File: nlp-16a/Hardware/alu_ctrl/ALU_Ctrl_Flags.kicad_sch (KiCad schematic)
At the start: 18 parts, among them U1 CD74HC00, U10 CD74HC00, U11 CD74HC00, U12 CD74HC00, U13 CD74HC00, U14 CD74HC00, U15 CD74HC00, U16 CD74HC00, U17 CD74HC00, U18 CD74HC00, U2 CD74HC00, U3 CD74HC00, U4 CD74HC00, U5 CD74HC00, U6 CD74HC00, U7 CD74HC00, U8 CD74HC00, U9 CD74HC00

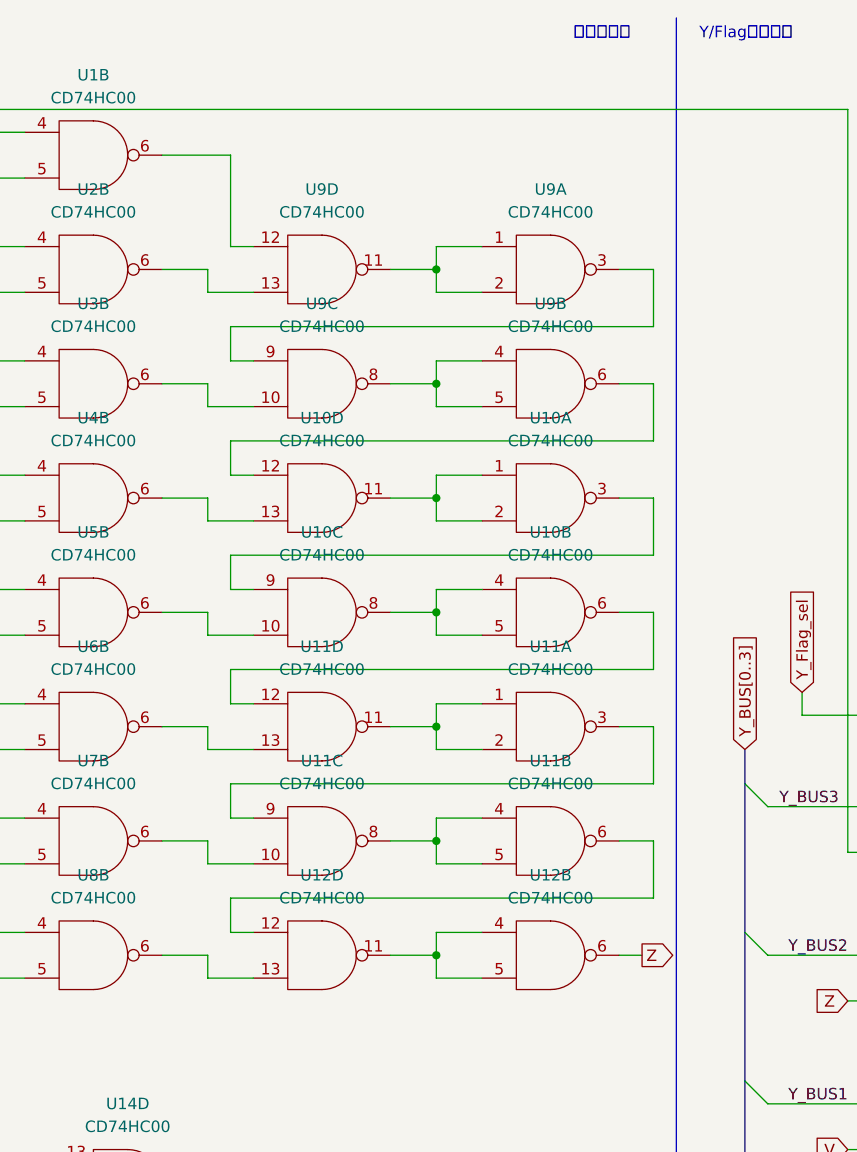
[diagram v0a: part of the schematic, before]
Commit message: ゼロフラグ高速化
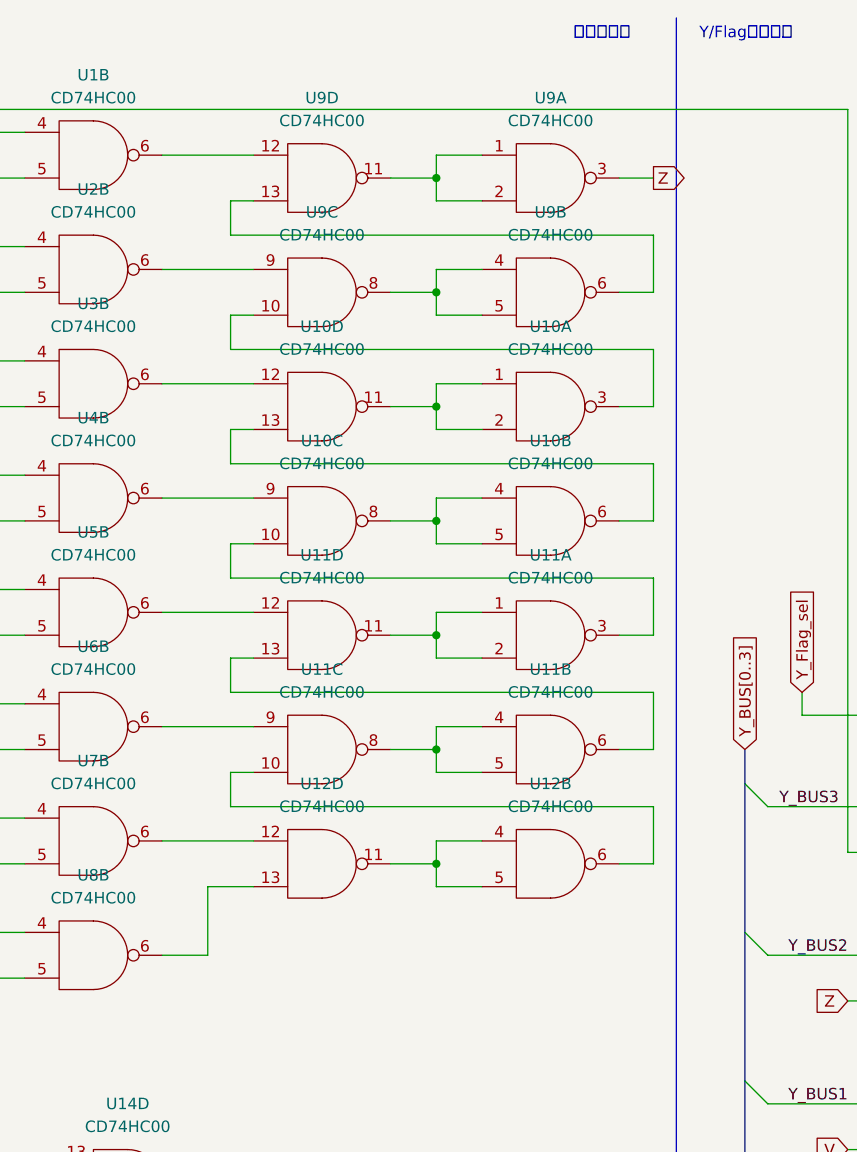
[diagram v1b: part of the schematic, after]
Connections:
- net Z: now also U9.3; no longer U12.6
- net at U9.13: now also U9.6; no longer U2.6
- net at U10.12: now also U3.6; no longer U9.6
- net at U10.13: now also U10.6; no longer U4.6
- net at U11.10: now also U12.6; no longer U7.6
- net at U11.9: now also U6.6; no longer U11.3
- net at U9.9: now also U2.6; no longer U9.3
- net at U12.12: now also U7.6; no longer U11.6
- net at U11.13: now also U11.6; no longer U6.6
- net at U11.12: now also U5.6; no longer U10.6
- net at U9.10: now also U10.3; no longer U3.6
- net at U10.10: now also U11.3; no longer U5.6
- net at U10.9: now also U4.6; no longer U10.3
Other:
- moved on the sheet: U10A, U10B, U10C, U10D, U11A, U11B, U11C, U11D, U12B, U12D, U9A, U9B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
